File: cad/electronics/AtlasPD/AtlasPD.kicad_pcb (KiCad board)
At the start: 2 copper layers, 39.6 x 19.1 mm, 16 parts, among them J1 Conn_01x02_Male, J2 Conn_01x02_Male, U1 LM2678T-ADJ_NOPB

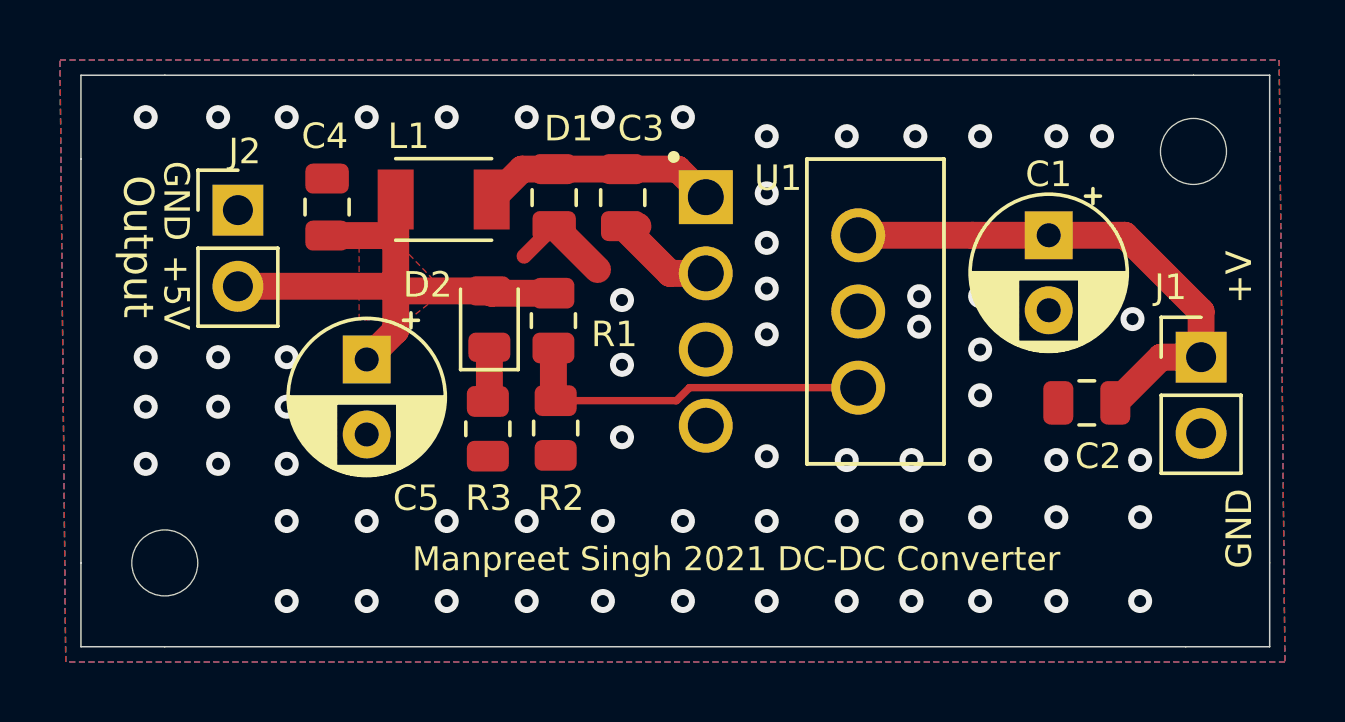
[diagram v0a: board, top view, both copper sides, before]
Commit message: More PCB changes
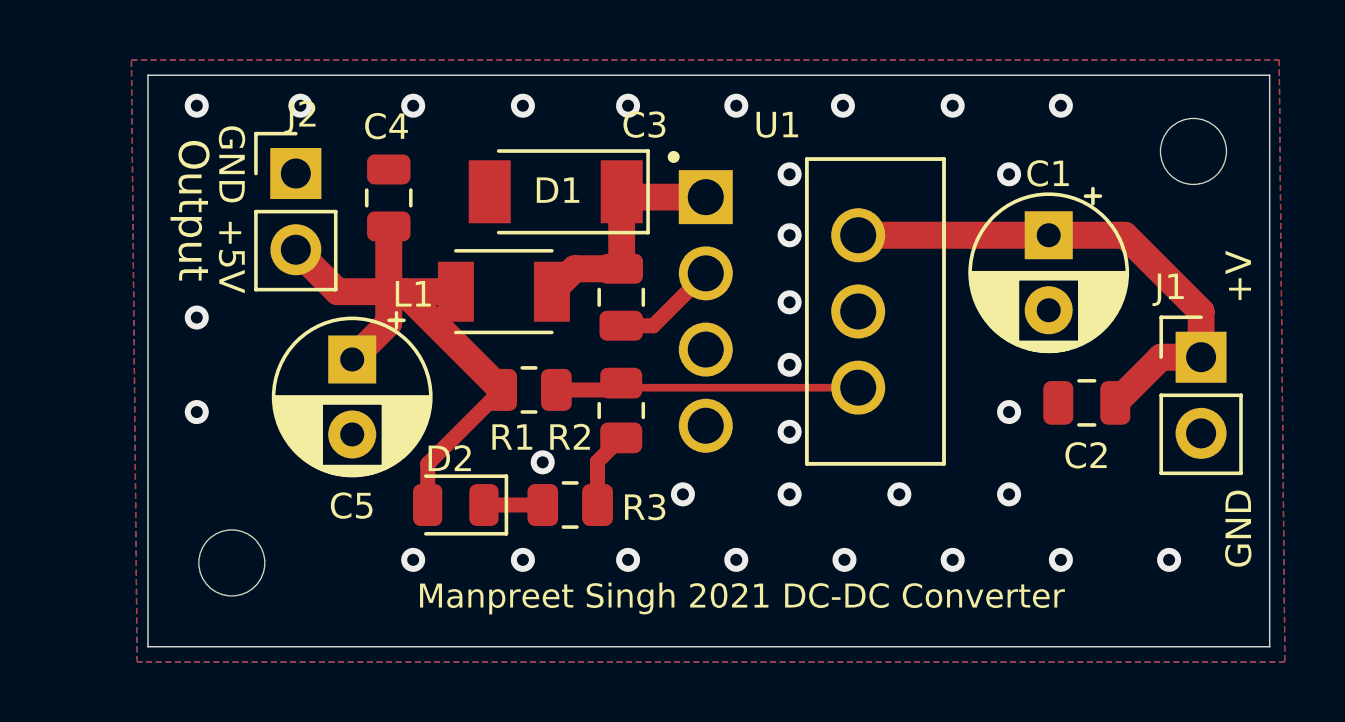
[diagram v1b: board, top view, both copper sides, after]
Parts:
- D1: footprint Capacitor_SMD:C_0805_2012Metric -> Diode_SMD:D_SOD-128
- moved D2 6.30 mm to (32.3, 32.4), turned to 180 degrees
- moved R3 3.74 mm to (36.1, 32.4), turned to 0 degrees
- moved L1 3.67 mm to (33.9, 25.2)
- moved C3 3.32 mm to (37.8, 25.4)
- moved R1 2.45 mm to (34.7, 28.5), turned to 0 degrees
- moved J2 2.28 mm to (27.0, 21.3)
- moved R2 2.26 mm to (37.8, 29.2)
- moved REF** 2.24 mm to (24.8, 34.3)
- moved C4 2.08 mm to (30.1, 22.1)
- moved C5 0.48 mm to (28.9, 27.5)
- moved D1 0.20 mm to (35.6, 21.9), turned to 180 degrees
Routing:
- net /Sheet60A23886/Output: track 18.6 -> 20.9 mm
- net Net-(R1-Pad2): track 12.1 -> 10.2 mm
- net GND: track 3.47 -> 2.56 mm, vias 66 -> 31
- removed copper zone on F.Cu, net /Sheet60A23886/Output
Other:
- board size 39.6 x 19.1 mm -> 37.4 x 19.1 mm
